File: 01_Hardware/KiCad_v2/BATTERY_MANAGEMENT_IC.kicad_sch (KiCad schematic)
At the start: 38 parts, among them J300 JST_B2B, Q300 BSS314PEH6327, Q301 IRLML2402TRPBF, U300 BQ25892

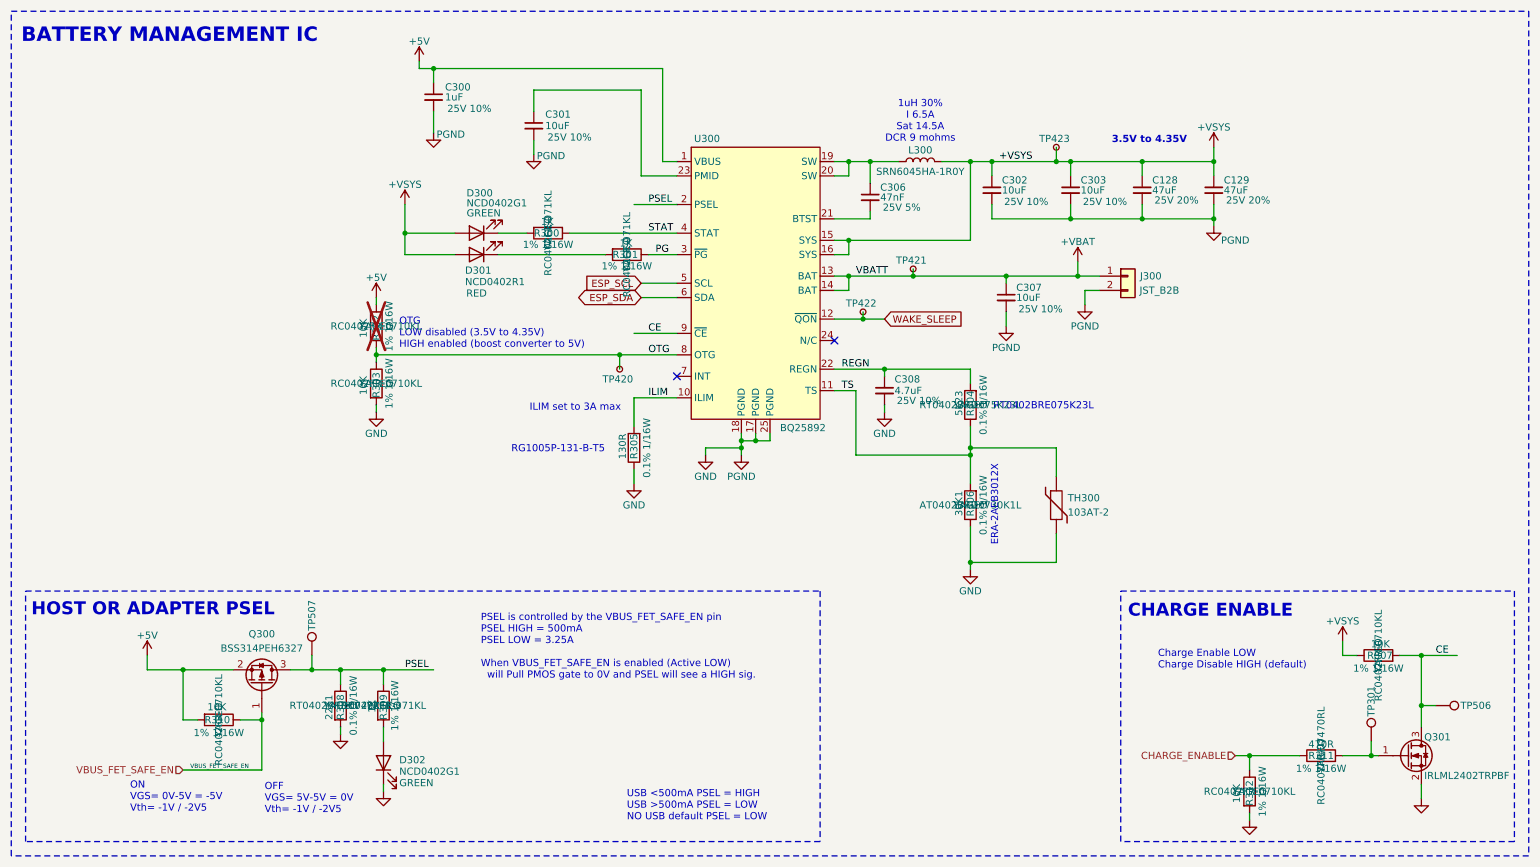
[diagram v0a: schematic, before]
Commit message: USB-C and Serial PCB routing done
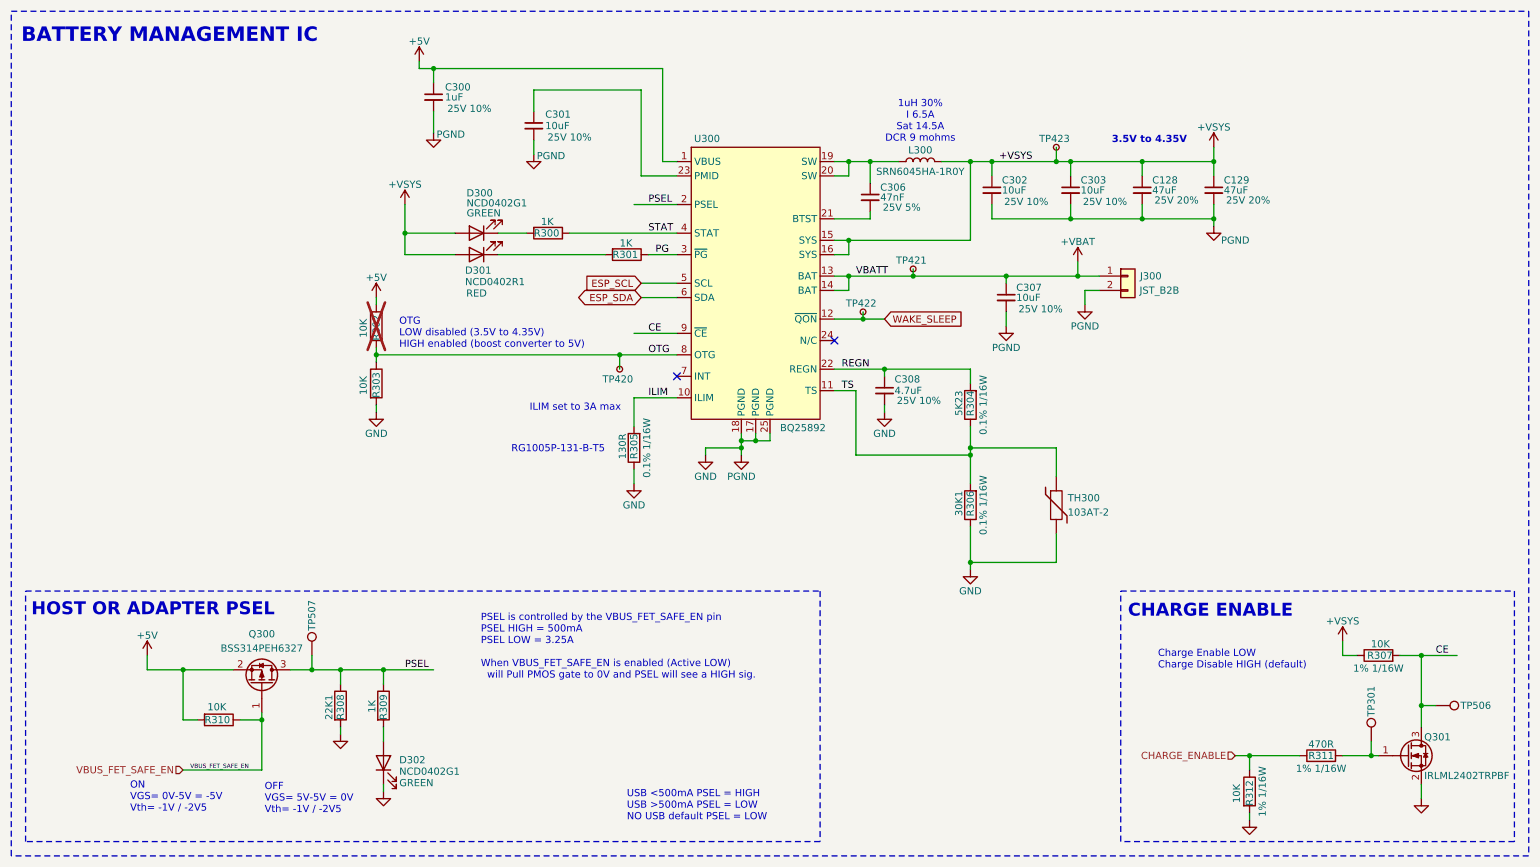
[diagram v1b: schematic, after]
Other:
- note removed: "ERA-2AEB3012X"
- note removed: "RT0402BRE075K23L"
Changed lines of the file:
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@@
 		)
 	)
-	(text "RT0402BRE075K23L"
-		(exclude_from_sim no)
-		(at 197.104 84.074 0)
-		(effects
-			(font
-				(size 1.27 1.27)
-			)
-		)
-	)
 	(text "PSEL is controlled by the VBUS_FET_SAFE_EN pin\nPSEL HIGH = 500mA\nPSEL LOW = 3.25A\n\nWhen VBUS_FET_SAFE_EN is enabled (Active LOW)\n  will Pull PMOS gate to 0V and PSEL will see a HIGH sig."
 		(exclude_from_sim no)
@@
 		)
 	)
-	(text "ERA-2AEB3012X"
-		(exclude_from_sim no)
-		(at 188.468 101.6 90)
-		(effects
-			(font
-				(size 1.27 1.27)
-			)
-		)
-	)
 	(text "ON\nVGS= 0V-5V = -5V\nVth= -1V / -2V5"
 		(exclude_from_sim no)
@@
 					(size 1.27 1.27)
 				)
+				(hide yes)
 			)
 		)
@@
 					(size 1.27 1.27)
 				)
+				(hide yes)
 			)
 		)
@@
 					(size 1.27 1.27)
 				)
+				(hide yes)
 			)
 		)
@@
 					(size 1.27 1.27)
 				)
+				(hide yes)
 			)
 		)
@@
 					(size 1.27 1.27)
 				)
+				(hide yes)
 			)
 		)
@@
 					(size 1.27 1.27)
 				)
+				(hide yes)
 			)
 		)
@@
 					(size 1.27 1.27)
 				)
+				(hide yes)
 			)
 		)
@@
 					(size 1.27 1.27)
 				)
+				(hide yes)
 			)
 		)
@@
 					(size 1.27 1.27)
 				)
+				(hide yes)
 			)
 		)
@@
 					(size 1.27 1.27)
 				)
+				(hide yes)
 			)
 		)
@@
 					(size 1.27 1.27)
 				)
+				(hide yes)
 			)
 		)
@@
 					(size 1.27 1.27)
 				)
+				(hide yes)
 			)
 		)
@@
 					(size 1.27 1.27)
 				)
+				(hide yes)
 			)
 		)
@@
 					(size 1.27 1.27)
 				)
+				(hide yes)
 			)
 		)
@@
 					(size 1.27 1.27)
 				)
+				(hide yes)
 			)
 		)
@@
 					(size 1.27 1.27)
 				)
+				(hide yes)
 			)
 		)
@@
 					(size 1.27 1.27)
 				)
+				(hide yes)
 			)
 		)
@@
 					(size 1.27 1.27)
 				)
+				(hide yes)
 			)
 		)
@@
 					(size 1.27 1.27)
 				)
+				(hide yes)
 			)
 		)
@@
 					(size 1.27 1.27)
 				)
+				(hide yes)
 			)
 		)
@@
 					(size 1.27 1.27)
 				)
+				(hide yes)
 			)
 		)
@@
 					(size 1.27 1.27)
 				)
+				(hide yes)
 			)
 		)
@@
 					(size 1.27 1.27)
 				)
+				(hide yes)
 			)
 		)
@@
 					(size 1.27 1.27)
 				)
+				(hide yes)
 			)
 		)
@@
 					(size 1.27 1.27)
 				)
+				(hide yes)
 			)
 		)
@@
 					(size 1.27 1.27)
 				)
+				(hide yes)
 			)
 		)
@@
 					(size 1.27 1.27)
 				)
+				(hide yes)
 			)
 		)
@@
 					(size 1.27 1.27)
 				)
+				(hide yes)
 			)
 		)
@@
 					(size 1.27 1.27)
 				)
+				(hide yes)
 			)
 		)
@@
 					(size 1.27 1.27)
 				)
+				(hide yes)
 			)
 		)
@@
 					(size 1.27 1.27)
 				)
+				(hide yes)
 			)
 		)
@@
 					(size 1.27 1.27)
 				)
+				(hide yes)
 			)
 		)
@@
 					(size 1.27 1.27)
 				)
+				(hide yes)
 			)
 		)
@@
 					(size 1.27 1.27)
 				)
+				(hide yes)
 			)
 		)
@@
 					(size 1.27 1.27)
 				)
+				(hide yes)
 			)
 		)
@@
 					(size 1.27 1.27)
 				)
+				(hide yes)
 			)
 		)
@@
 					(size 1.27 1.27)
 				)
+				(hide yes)
 			)
 		)
@@
 					(size 1.27 1.27)
 				)
+				(hide yes)
 			)
 		)
@@
 					(size 1.27 1.27)
 				)
+				(hide yes)
 			)
 		)
@@
 					(size 1.27 1.27)
 				)
+				(hide yes)
 			)
 		)
@@
 					(size 1.27 1.27)
 				)
+				(hide yes)
 			)
 		)
@@
 					(size 1.27 1.27)
 				)
+				(hide yes)
 			)
 		)
@@
 					(size 1.27 1.27)
 				)
+				(hide yes)
 			)
 		)
@@
 					(size 1.27 1.27)
 				)
+				(hide yes)
 			)
 		)
@@
 					(size 1.27 1.27)
 				)
+				(hide yes)
 			)
 		)
@@
 					(size 1.27 1.27)
 				)
+				(hide yes)
 			)
 		)
@@
 					(size 1.27 1.27)
 				)
+				(hide yes)
 			)
 		)
@@
 					(size 1.27 1.27)
 				)
+				(hide yes)
 			)
 		)
@@
 					(size 1.27 1.27)
 				)
+				(hide yes)
 			)
 		)
@@
 					(size 1.27 1.27)
 				)
+				(hide yes)
 			)
 		)
@@
 					(size 1.27 1.27)
 				)
+				(hide yes)
 			)
 		)
@@
 					(size 1.27 1.27)
 				)
+				(hide yes)
 			)
 		)
@@
 					(size 1.27 1.27)
 				)
+				(hide yes)
 			)
 		)
@@
 					(size 1.27 1.27)
 				)
+				(hide yes)
 			)
 		)
@@
 					(size 1.27 1.27)
 				)
+				(hide yes)
 			)
 		)
